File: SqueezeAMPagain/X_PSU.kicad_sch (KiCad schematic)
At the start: 1 part, among them J10 Conn_02x07_Odd_Even

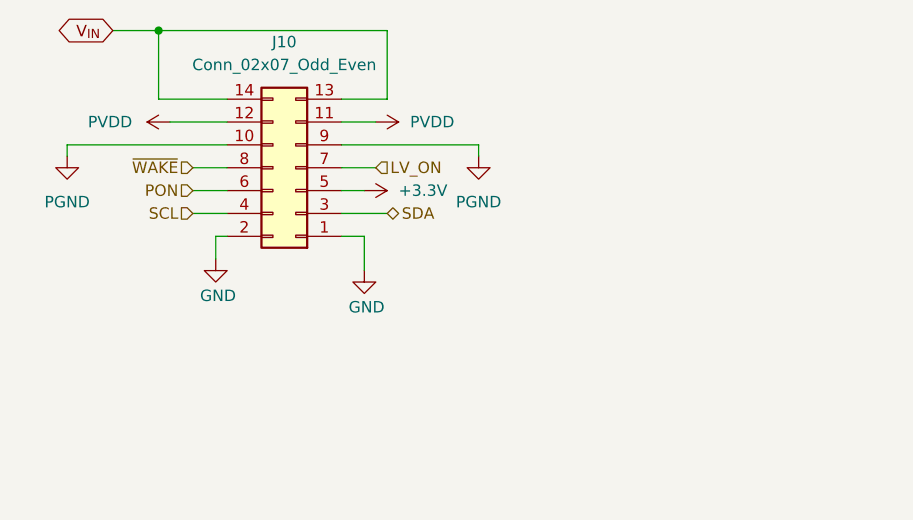
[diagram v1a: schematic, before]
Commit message: Update SqueezeAMPagain.kicad_pcb, SqueezeAMPagain.kicad_prl, SqueezeAMPagain.kicad_pro, and 4 more files
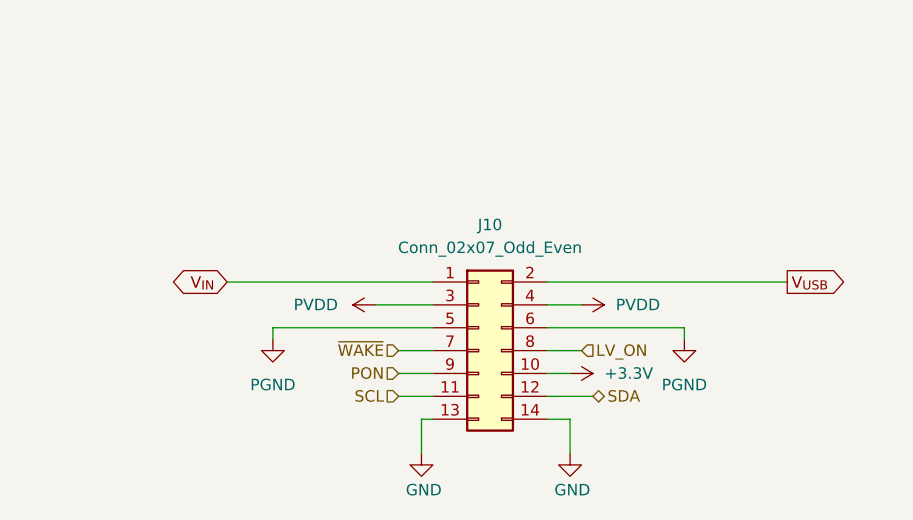
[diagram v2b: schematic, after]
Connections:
- net +3.3V: now also J10.10 (Pin_10); no longer J10.5 (Pin_5)
- net GND: now also J10.13 (Pin_13), J10.14 (Pin_14); no longer J10.1 (Pin_1), J10.2 (Pin_2)
- net LV_ON: now also J10.8 (Pin_8); no longer J10.7 (Pin_7)
- net PGND: now also J10.5 (Pin_5), J10.6 (Pin_6); no longer J10.10 (Pin_10), J10.9 (Pin_9)
- net PON: now also J10.9 (Pin_9); no longer J10.6 (Pin_6)
- net PVDD: now also J10.3 (Pin_3), J10.4 (Pin_4); no longer J10.11 (Pin_11), J10.12 (Pin_12)
- net SCL: now also J10.11 (Pin_11); no longer J10.4 (Pin_4)
- net SDA: now also J10.12 (Pin_12); no longer J10.3 (Pin_3)
- net V_{IN}: now also J10.1 (Pin_1); no longer J10.13 (Pin_13), J10.14 (Pin_14)
- net ~{WAKE}: now also J10.7 (Pin_7); no longer J10.8 (Pin_8)
- new net V_{USB}: J10.2 (Pin_2)
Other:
- moved on the sheet: J10
